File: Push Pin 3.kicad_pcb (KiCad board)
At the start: 2 copper layers, 92 x 75.9 mm, 34 parts, among them J1 Screw_Terminal_01x02, J2 Screw_Terminal_01x02, J3 Screw_Terminal_01x02, J4 Screw_Terminal_01x02, J5 Screw_Terminal_01x02, J6 Screw_Terminal_01x02, J7 Screw_Terminal_01x02, Q1 NTR4101PT1G, Q2 NTR4101PT1G, Q3 NTR4101PT1G, SW4 SW_DPDT_x2, SW5 SW_DPDT_x2, SW6 SW_DPDT_x2, U2 LDO_4v2-MIC5209-4.2YS-TR

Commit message: Plus beau
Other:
- board text added: "+"
- board text added: "-"
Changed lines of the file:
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@@
 		)
 		(fp_text user "+"
-			(at 14.5 -2.595 90)
+			(at 10 -0.5 90)
 			(layer "B.SilkS")
 			(effects
@@
 		)
 	)
+	(gr_text "-"
+		(at 139.5 113 0)
+		(layer "B.SilkS")
+		(effects
+			(font
+				(size 1.5 1.5)
+				(thickness 0.15)
+			)
+			(justify left bottom)
+		)
+	)
 	(gr_text "ODB1\n3v7\n"
 		(at 185.4798 84.2549 0)
@@
 		)
 	)
+	(gr_text "+"
+		(at 168.5 129.5 0)
+		(layer "B.SilkS")
+		(effects
+			(font
+				(size 1.5 1.5)
+				(thickness 0.15)
+			)
+			(justify left bottom)
+		)
+	)
 	(gr_text "Easymini"
 		(at 137.5 114.5 0)
@@
 	)
 	(gr_text "9V"
-		(at 142 114 0)
+		(at 146 113 0)
 		(layer "B.SilkS")
 		(effects
@@
 		)
 	)
+	(gr_text "+"
+		(at 140 100 0)
+		(layer "B.SilkS")
+		(effects
+			(font
+				(size 1.5 1.5)
+				(thickness 0.15)
+			)
+			(justify left bottom)
+		)
+	)
+	(gr_text "+"
+		(at 132.5 100 0)
+		(layer "B.SilkS")
+		(effects
+			(font
+				(size 1.5 1.5)
+				(thickness 0.15)
+			)
+			(justify left bottom)
+		)
+	)

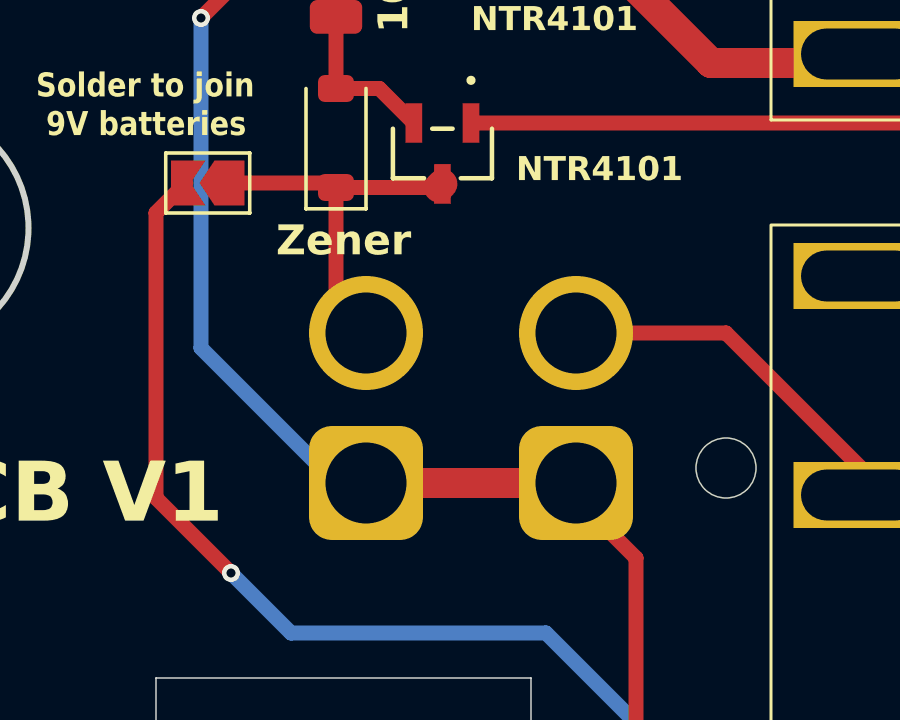
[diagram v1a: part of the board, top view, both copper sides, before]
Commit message: touch up
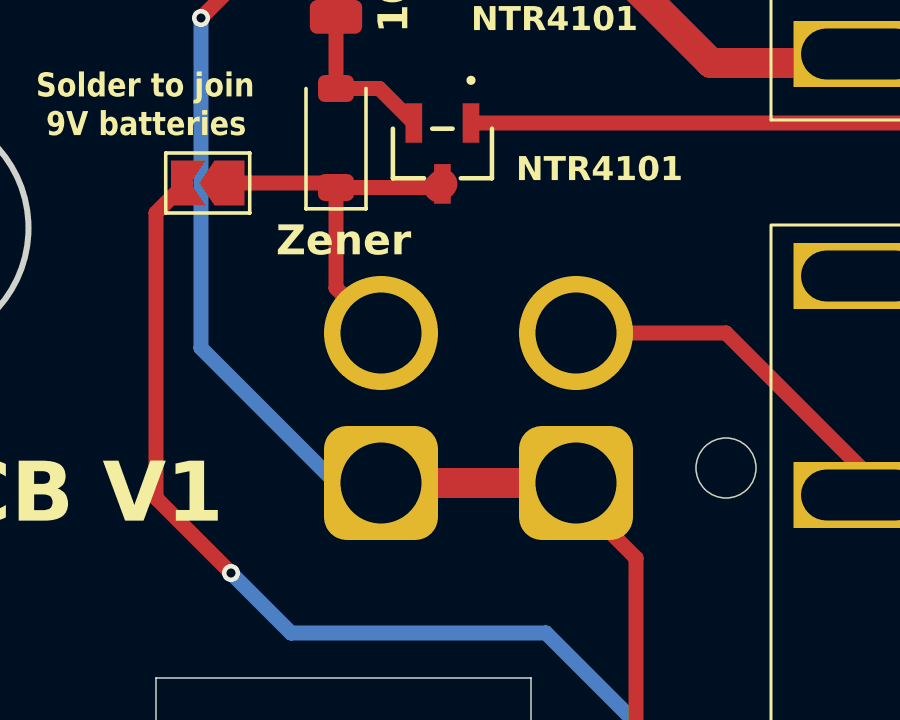
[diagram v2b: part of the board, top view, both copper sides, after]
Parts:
- moved J3 0.50 mm to (134.0, 108.5)
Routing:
- net Net-(DZ3-K): track 12.5 -> 13.2 mm
- net Net-(Batt_7v2-Pin_1): track 45.2 -> 45.7 mm
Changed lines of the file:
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@@
 	(footprint "Connector_AMASS:AMASS_XT30U-M_1x02_P5.0mm_Vertical"
 		(layer "B.Cu")
-		(at 133.5 108.5 90)
+		(at 134 108.5 90)
 		(descr "Connector XT30 Vertical Cable Male, https://www.tme.eu/Document/7d9d972ae3468777f69ec2ee99897652/XT30U-M.pdf")
 		(tags "RC Connector XT30")
@@
 	)
 	(segment
-		(start 132.5 108.5)
-		(end 140 108.5)
+		(start 134 108.5)
+		(end 140.5 108.5)
 		(width 1)
 		(layer "F.Cu")
@@
 	)
 	(segment
+		(start 132.5 108.5)
+		(end 134 108.5)
+		(width 0.5)
+		(layer "B.Cu")
+		(net 6)
+	)
+	(segment
 		(start 128 104)
 		(end 132.5 108.5)
@@
 	)
 	(segment
-		(start 133.5 103.5)
-		(end 132.5 102.5)
+		(start 132.5 102)
+		(end 132.5 98.65)
 		(width 0.5)
 		(layer "F.Cu")
@@
 	)
 	(segment
-		(start 132.35 98.5)
-		(end 132.5 98.65)
+		(start 134 103.5)
+		(end 132.5 102)
 		(width 0.5)
 		(layer "F.Cu")
@@
 	)
 	(segment
-		(start 128.95 98.5)
-		(end 132.35 98.5)
+		(start 133.5 103.5)
+		(end 134 103.5)
 		(width 0.5)
 		(layer "F.Cu")
@@
 	)
 	(segment
-		(start 132.5 102.5)
+		(start 132.35 98.5)
 		(end 132.5 98.65)
 		(width 0.5)
 		(layer "F.Cu")
+		(net 14)
+	)
+	(segment
+		(start 128.95 98.5)
+		(end 132.35 98.5)
+		(width 0.5)
+		(layer "F.Cu")
